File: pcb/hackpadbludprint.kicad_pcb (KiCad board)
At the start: 2 copper layers, 32.6 x 98.7 mm, 6 parts, among them SW1 SW_Push, SW2 SW_Push, SW3 SW_Push, SW4 SW_Push, U1 MOUDLE-SEEEDUINO-XIAO

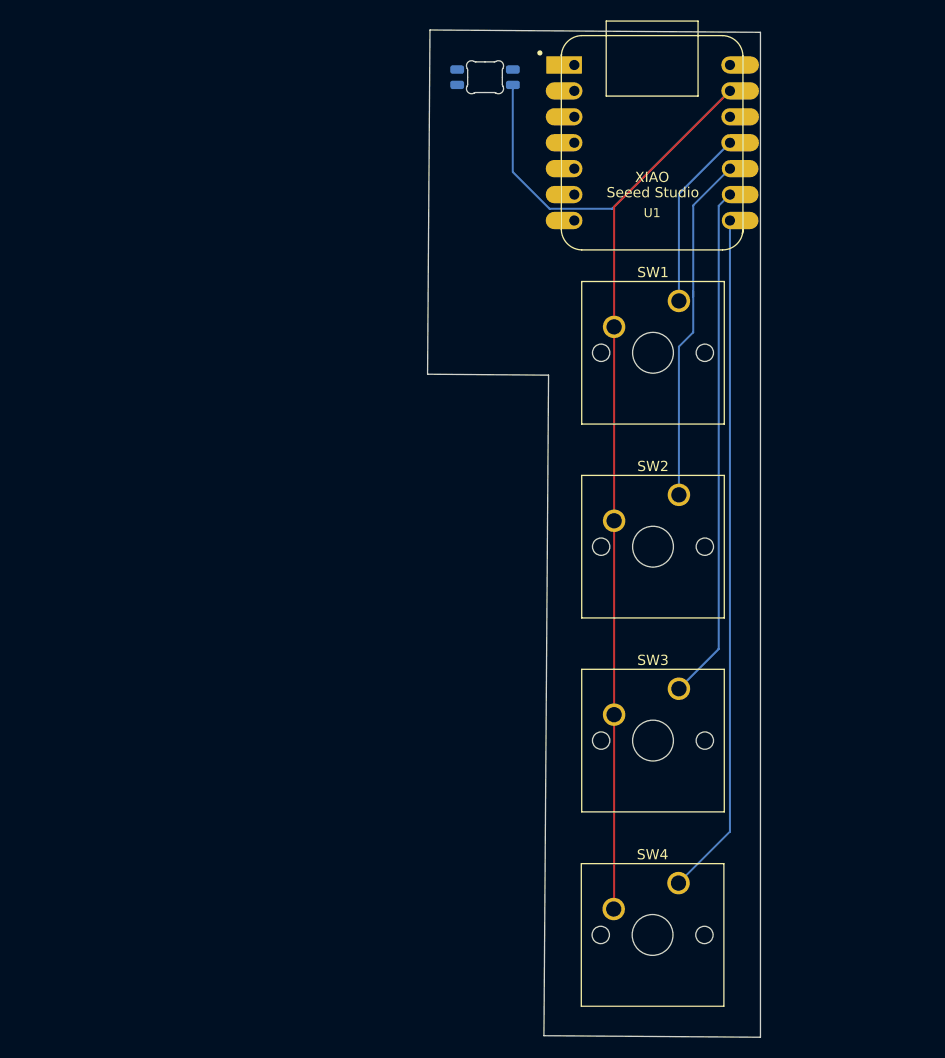
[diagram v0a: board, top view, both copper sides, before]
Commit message: STRETCH 3!!!!
- board looking nice
- Tysm jame
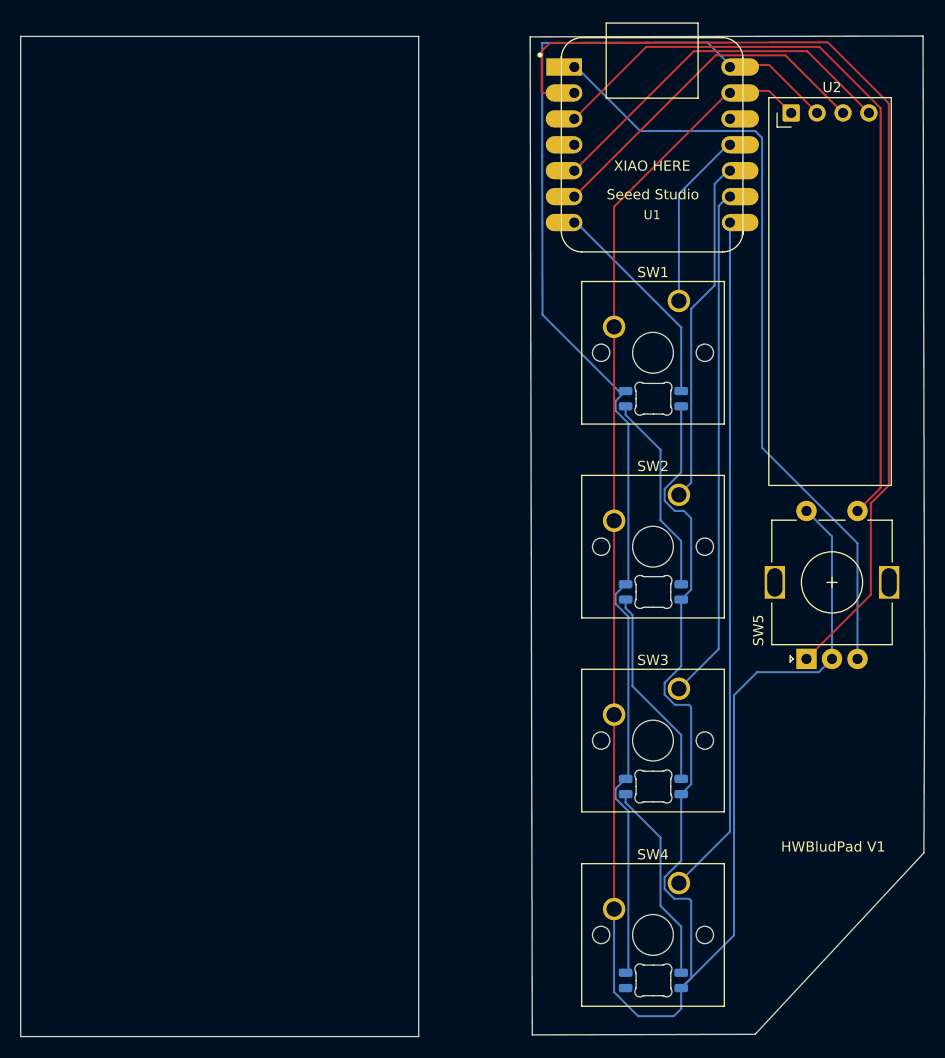
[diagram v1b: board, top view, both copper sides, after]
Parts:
- added D2: SK6812MINI-E, LED_SMD:LED_SK6812MINI-E_3.2x2.8mm_P1.5mm_ReverseMount, B.Cu at (150.5, 104.4)
- added D3: SK6812MINI-E, LED_SMD:LED_SK6812MINI-E_3.2x2.8mm_P1.5mm_ReverseMount, B.Cu at (150.5, 123.5)
- added D4: SK6812MINI-E, LED_SMD:LED_SK6812MINI-E_3.2x2.8mm_P1.5mm_ReverseMount, B.Cu at (150.5, 142.5)
- added SW5: RotaryEncoder_Switch, Rotary_Encoder:RotaryEncoder_Alps_EC11E-Switch_Vertical_H20mm, F.Cu at (165.5, 111.0)
- added U2: ER_OLEDM0.91_1x-I2C, Display:ER_OLEDM0.91_1x-I2C, F.Cu at (164.0, 57.5)
- moved D1 35.6 mm to (150.5, 85.5)
- moved U1 0.20 mm to (150.4, 60.6)
- renumbered D2 to D1
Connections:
- D1 pad 2: Net-(D2-DIN) -> Net-(D1-DIN)
- U1 pad 1: unconnected-(U1-PA02_A0_D0-Pad1) -> Net-(U1-PA02_A0_D0)
- U1 pad 14: unconnected-(U1-5V-Pad14) -> +5V
- U1 pad 2: unconnected-(U1-PA4_A1_D1-Pad2) -> Net-(U1-PA4_A1_D1)
- U1 pad 3: unconnected-(U1-PA10_A2_D2-Pad3) -> Net-(U1-PA10_A2_D2)
- U1 pad 5: Net-(D2-DIN) -> Net-(U1-PA8_A4_D4_SDA)
- U1 pad 6: unconnected-(U1-PA9_A5_D5_SCL-Pad6) -> Net-(U1-PA9_A5_D5_SCL)
- U1 pad 7: unconnected-(U1-PB08_A6_D6_TX-Pad7) -> Net-(D1-DIN)
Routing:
- net +5V: track 0.00 -> 127.8 mm
- net GND: track 121.2 -> 233.2 mm
- net Net-(U1-PA4_A1_D1): track 0.00 -> 103.5 mm
- net Net-(U1-PA02_A0_D0): track 0.00 -> 76.3 mm
- net Net-(U1-PA10_A2_D2): track 0.00 -> 75.8 mm
- net Net-(U1-PA8_A4_D4_SDA): track 0.00 -> 36.2 mm
- net Net-(U1-PA9_A5_D5_SCL): track 0.00 -> 34.4 mm
- net Net-(D1-DIN): track 0.00 -> 21.0 mm
- net Net-(D2-DOUT): track 0.00 -> 19.8 mm
- net Net-(D3-DOUT): track 0.00 -> 19.8 mm
- net Net-(D1-DOUT): track 0.00 -> 19.7 mm
- net unconnected-(U1-PA4_A1_D1-Pad2): track 1.59 -> 0.00 mm
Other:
- board size 32.6 x 98.7 mm -> 88.6 x 98 mm
- board text added: "HWBludPad V1"
